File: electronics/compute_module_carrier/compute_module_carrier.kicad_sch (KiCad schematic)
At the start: 0 parts

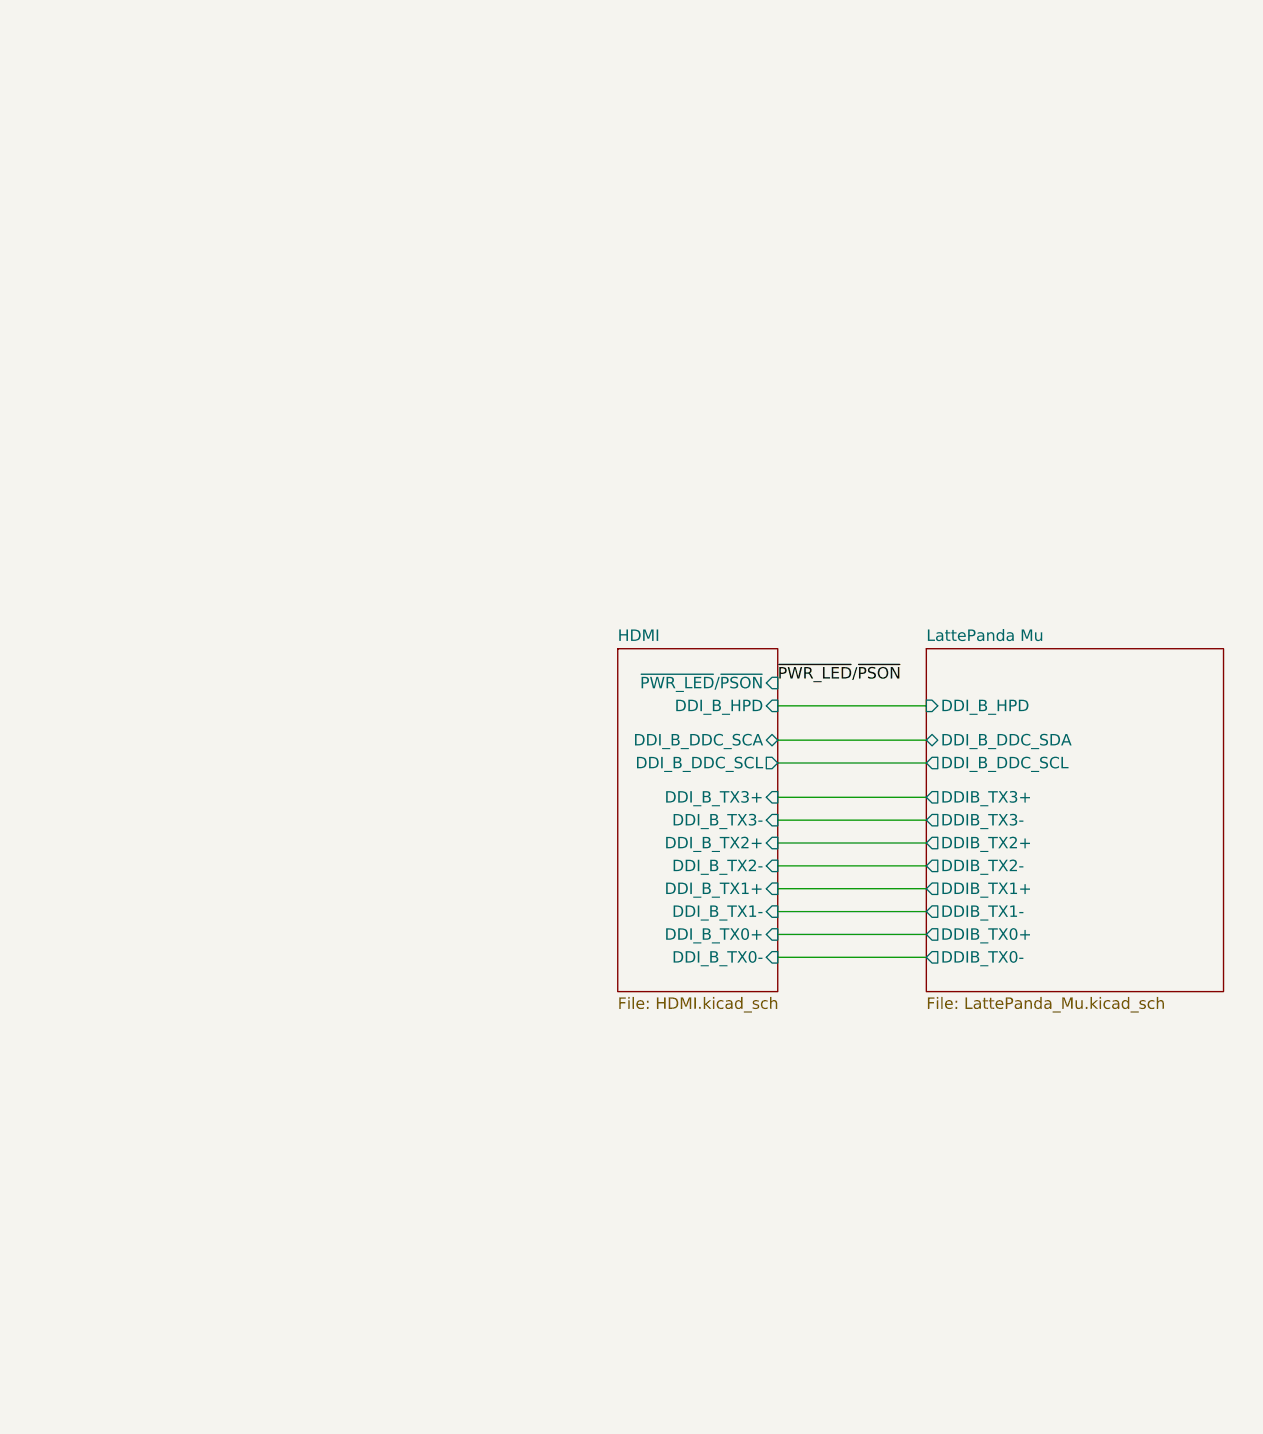
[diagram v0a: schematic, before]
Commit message: designing the compute module carrier pt.4
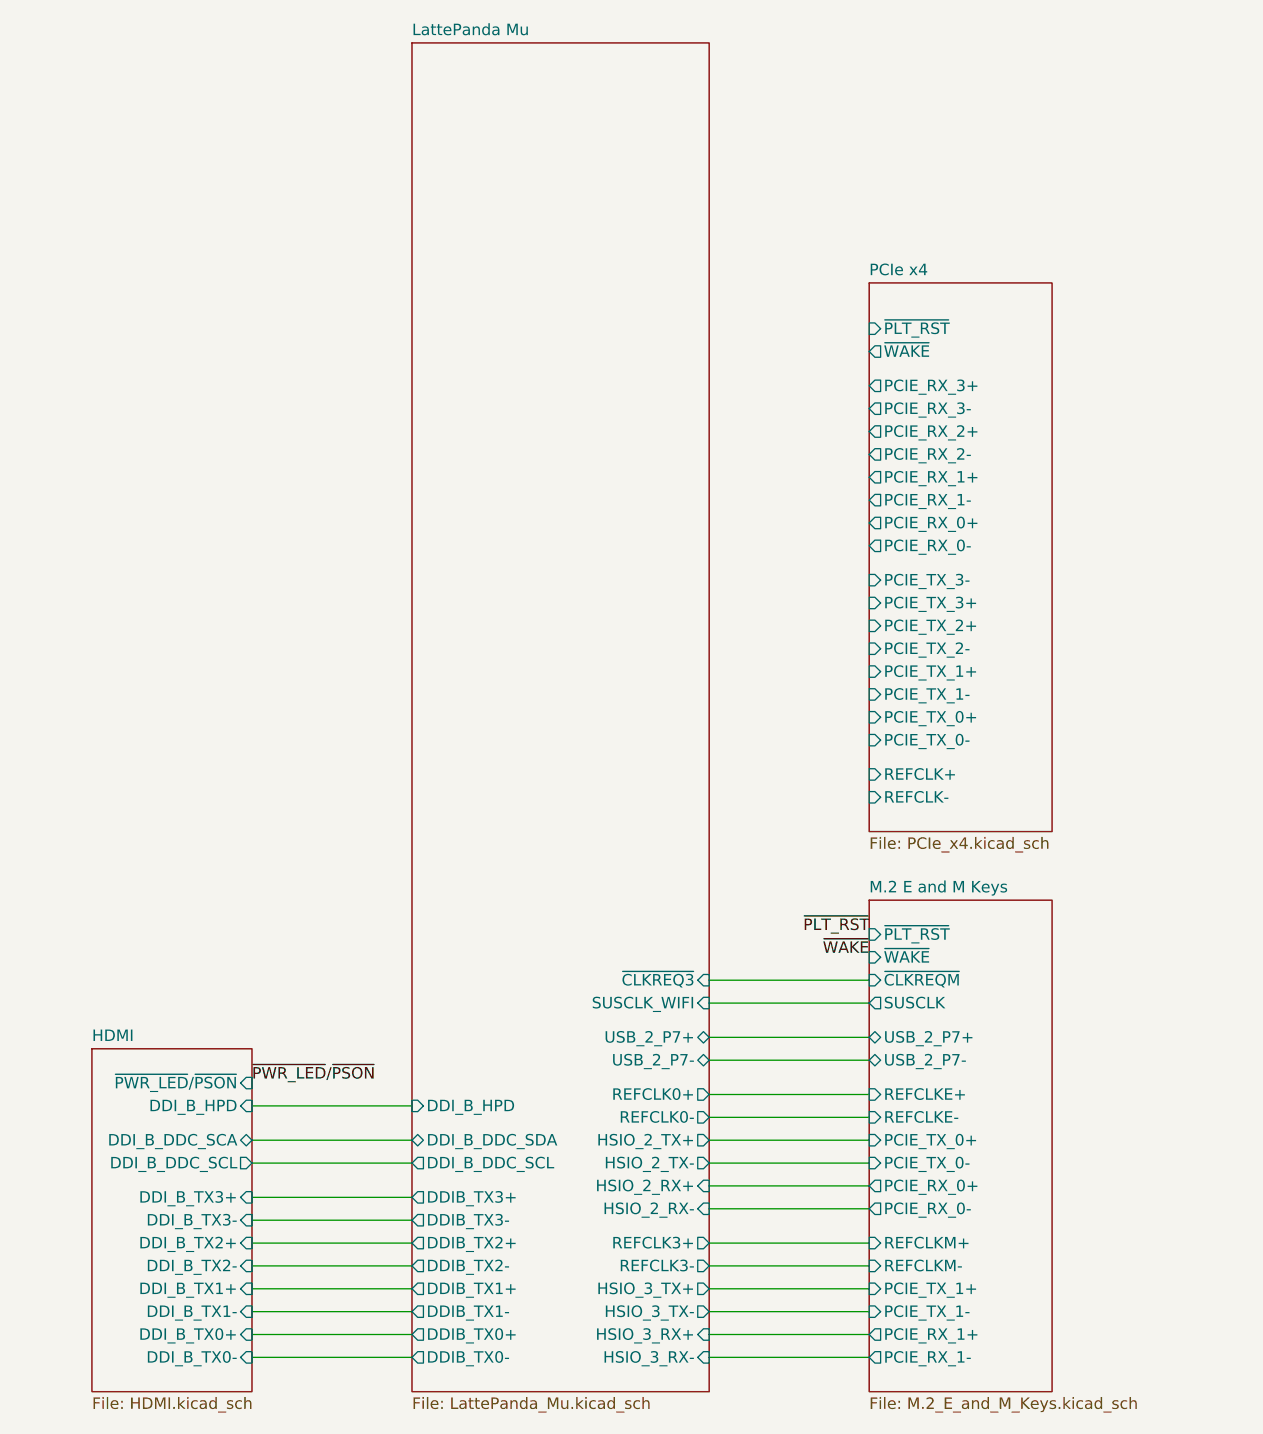
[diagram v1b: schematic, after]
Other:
- added sheet M.2 E and M Keys (M.2_E_and_M_Keys.kicad_sch)
- added sheet PCIe x4 (PCIe_x4.kicad_sch)
- sheet LattePanda Mu ports: added HSIO_2_RX+, HSIO_2_RX-, HSIO_2_TX+, HSIO_2_TX-, HSIO_3_RX+, HSIO_3_RX-, HSIO_3_TX+, HSIO_3_TX-, REFCLK0+, REFCLK0-, REFCLK3+, REFCLK3-, SUSCLK_WIFI, USB_2_P7+, USB_2_P7-, ~{CLKREQ3}; removed none
